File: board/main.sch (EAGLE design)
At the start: 63 parts, among them J1 HEADER4VALULOK, J2 HEADER6, J3 FUSE, Q1 MOSFET-NCHANNELTO-220-FLAT, Q2 MOSFET-NCHANNELTO-220-FLAT, Q3 MOSFET-NCHANNELTO-220-FLAT, Q4 MOSFET-NCHANNELTO-220-FLAT, Q5 MOSFET-NCHANNELTO-220-FLAT, Q6 MOSFET-NCHANNELTO-220-FLAT, U2 INA181, U3 TC1240A, U4 K78U05, U5 DGD2304, U6 DGD2304, U7 DGD2304

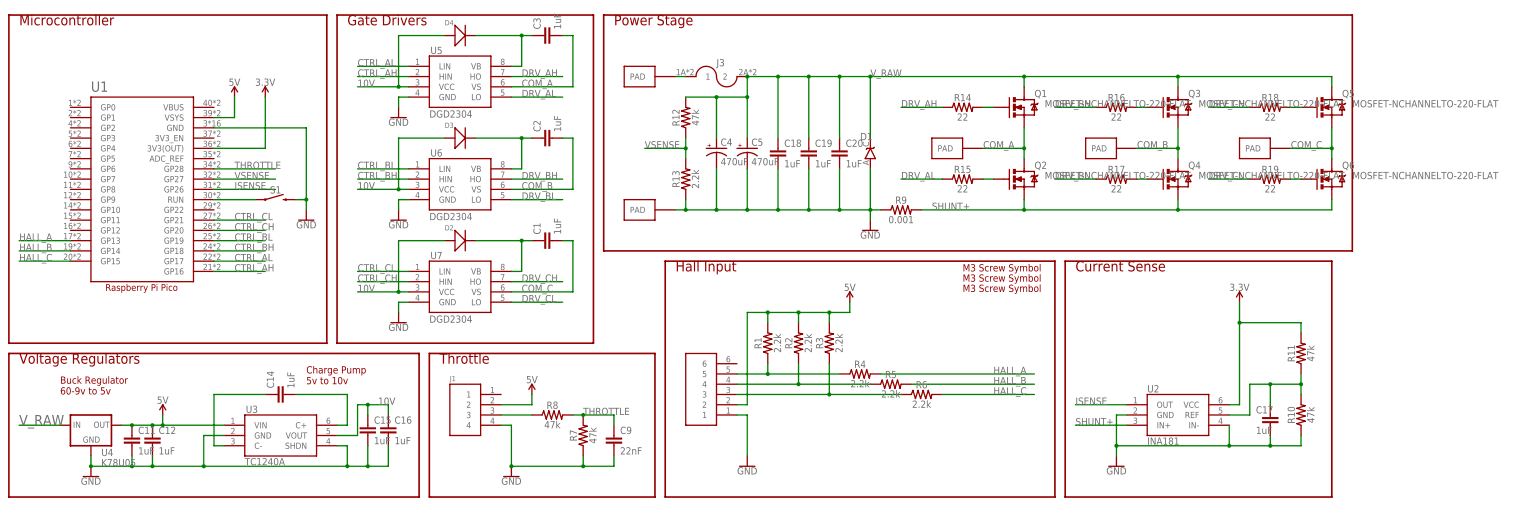
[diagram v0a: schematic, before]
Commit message: Code works
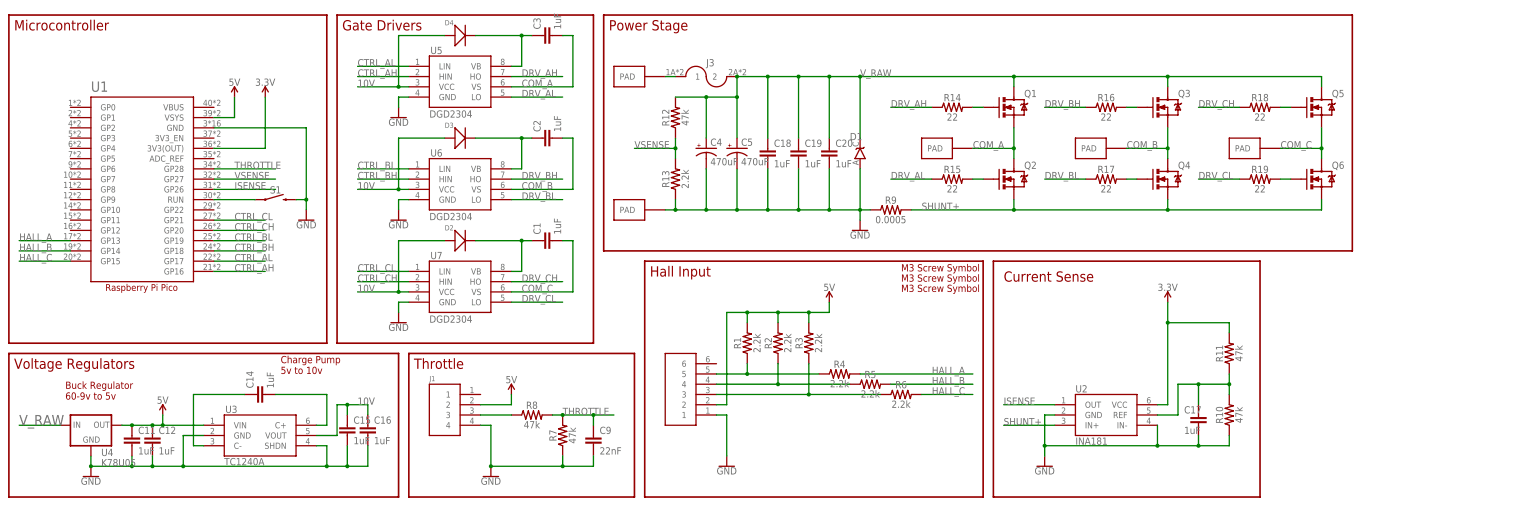
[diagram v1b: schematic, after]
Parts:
- R9: value 0.001 -> 0.0005
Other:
- moved on the sheet: C14, C15, C16, C17, C18, C19, C20, C4, C5, C9, D1, J1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
